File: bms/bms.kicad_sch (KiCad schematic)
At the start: 32 parts, among them J10 Conn_02x10_Odd_Even, J11 Conn_02x08_Odd_Even, J12 Conn_02x10_Odd_Even, J13 Conn_02x08_Odd_Even, J14 Conn_02x08_Odd_Even, J15 Conn_02x10_Odd_Even, J2 Conn_01x08_Socket, J3 Conn_01x06_Socket, J5 Conn_01x10_Socket, J6 Conn_01x08_Socket

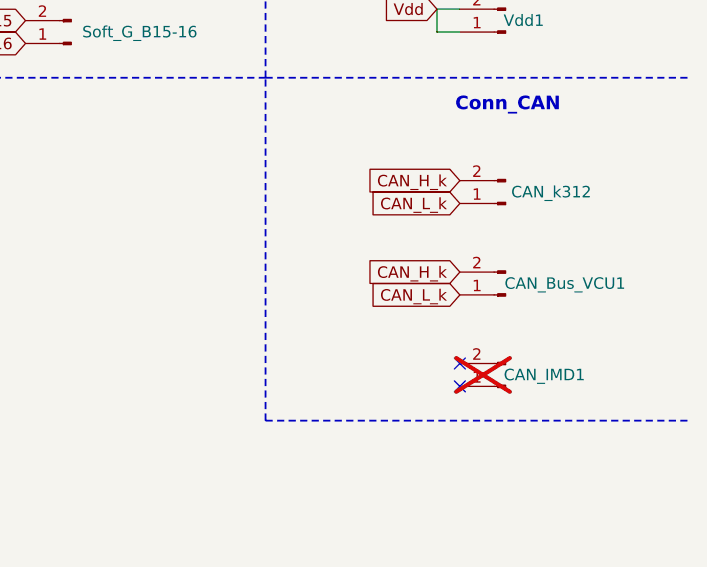
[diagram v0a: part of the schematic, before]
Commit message: inca un update
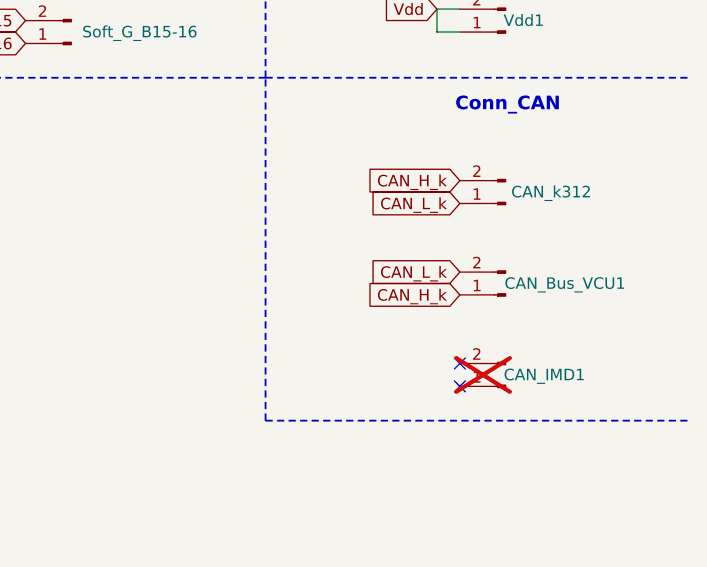
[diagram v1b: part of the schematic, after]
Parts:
- CAN_Bus_VCU1: footprint Connector_PinHeader_2.00mm:PinHeader_1x02_P2.00mm_Vertical -> Connector_JST:JST_PH_S2B-PH-K_1x02_P2.00mm_Horizontal
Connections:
- net CAN_H_k: now also CAN_Bus_VCU1.1 (Pin_1); no longer CAN_Bus_VCU1.2 (Pin_2)
- net CAN_L_k: now also CAN_Bus_VCU1.2 (Pin_2); no longer CAN_Bus_VCU1.1 (Pin_1)
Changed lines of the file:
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@@
 		)
 	)
-	(global_label "CAN_H_k"
-		(shape input)
-		(at 260.35 71.12 180)
-		(fields_autoplaced yes)
-		(effects
-			(font
-				(size 1.27 1.27)
-			)
-			(justify right)
-		)
-		(property "Intersheetrefs" "${INTERSHEET_REFS}"
-			(at 249.3819 71.12 0)
-			(effects
-				(font
-					(size 1.27 1.27)
-				)
-				(justify right)
-				(hide yes)
-			)
-		)
-	)
 	(global_label "CAN_L_k"
 		(shape input)
@@
 		)
 	)
+	(global_label "CAN_H_k"
+		(shape input)
+		(at 260.35 73.66 180)
+		(fields_autoplaced yes)
+		(effects
+			(font
+				(size 1.27 1.27)
+			)
+			(justify right)
+		)
+		(property "Intersheetrefs" "${INTERSHEET_REFS}"
+			(at 249.3819 73.66 0)
+			(effects
+				(font
+					(size 1.27 1.27)
+				)
+				(justify right)
+				(hide yes)
+			)
+		)
+	)
 	(global_label "4"
 		(shape input)
@@
 		)
 	)
+	(global_label "CAN_L_k"
+		(shape input)
+		(at 260.35 71.12 180)
+		(fields_autoplaced yes)
+		(effects
+			(font
+				(size 1.27 1.27)
+			)
+			(justify right)
+		)
+		(property "Intersheetrefs" "${INTERSHEET_REFS}"
+			(at 249.6843 71.12 0)
+			(effects
+				(font
+					(size 1.27 1.27)
+				)
+				(justify right)
+				(hide yes)
+			)
+		)
+	)
 	(global_label "3"
 		(shape input)
@@
 		)
 	)
-	(global_label "CAN_L_k"
-		(shape input)
-		(at 260.35 73.66 180)
-		(fields_autoplaced yes)
-		(effects
-			(font
-				(size 1.27 1.27)
-			)
-			(justify right)
-		)
-		(property "Intersheetrefs" "${INTERSHEET_REFS}"
-			(at 249.6843 73.66 0)
-			(effects
-				(font
-					(size 1.27 1.27)
-				)
-				(justify right)
-				(hide yes)
-			)
-		)
-	)
 	(global_label "G9"
 		(shape input)
@@
 			)
 		)
-		(property "Footprint" "Connector_PinHeader_2.00mm:PinHeader_1x02_P2.00mm_Vertical"
+		(property "Footprint" "Connector_JST:JST_PH_S2B-PH-K_1x02_P2.00mm_Horizontal"
 			(at 265.43 73.66 0)
 			(effects
